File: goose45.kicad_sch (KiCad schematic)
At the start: 25 parts, among them SW1 Conn_01x02_Female, SW2 SW_Push, U1 STM32F103CBTx, X1 Crystal_GND24

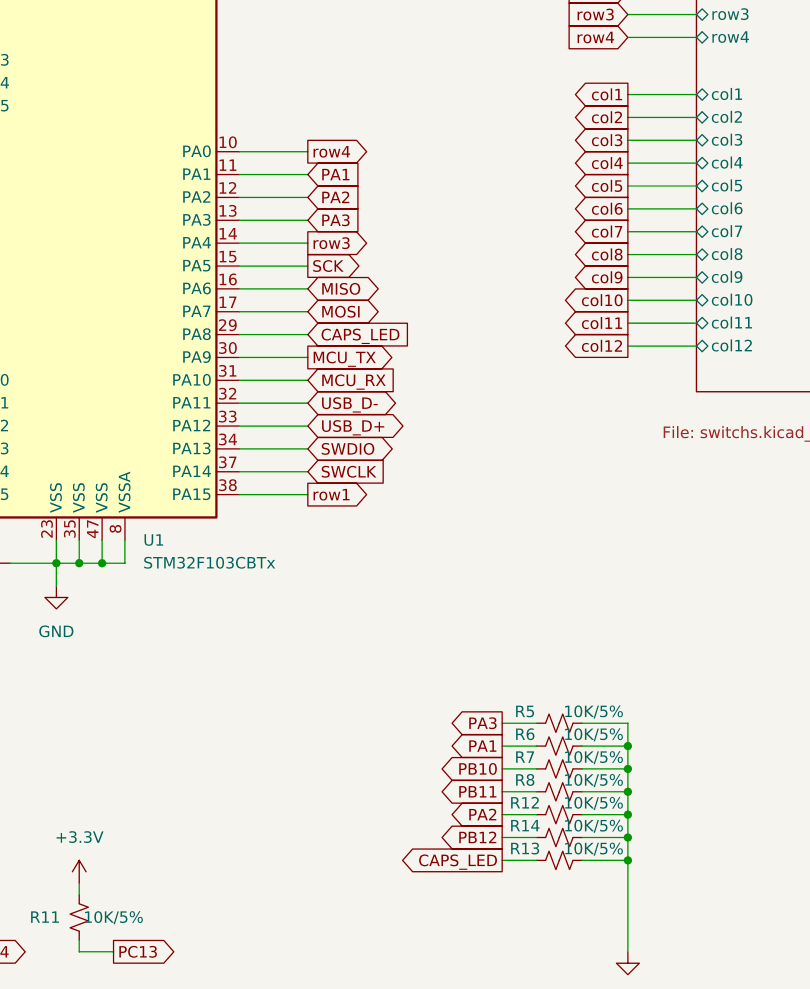
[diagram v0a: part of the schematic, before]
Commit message: update PCB layout
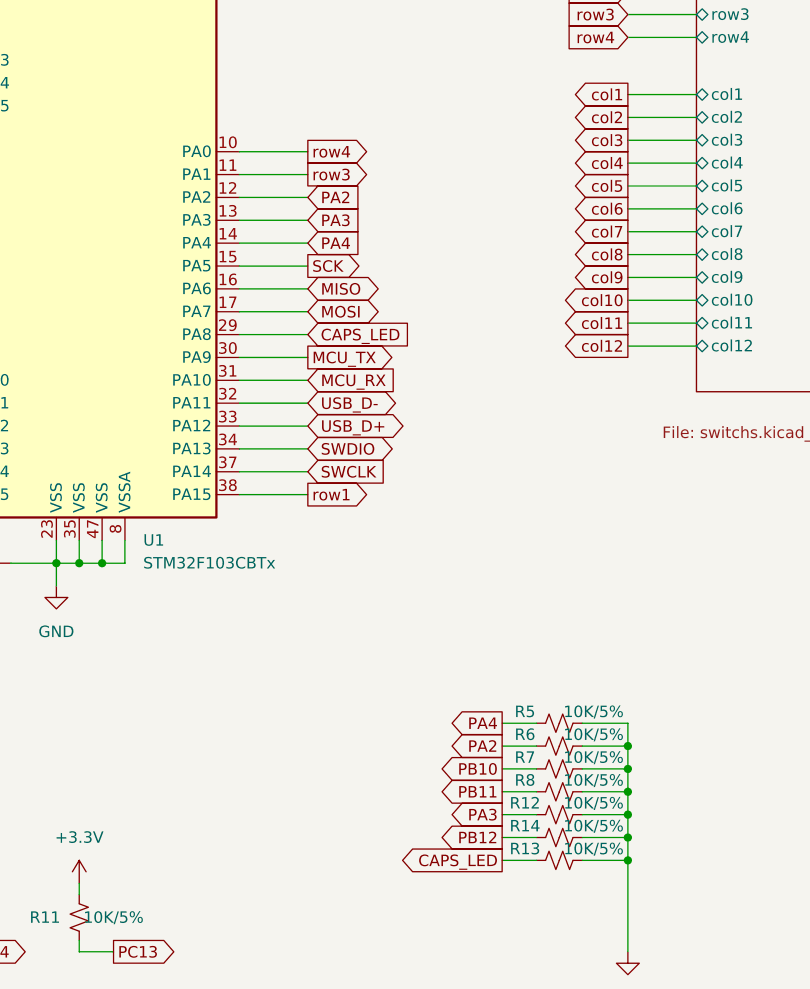
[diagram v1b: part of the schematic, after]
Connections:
- net PA2: now also R6.2; no longer R12.2
- net PA3: now also R12.2; no longer R5.2
- net row3: now also U1.11 (PA1); no longer U1.14 (PA4)
- removed net PA1: R6.2, U1.11 (PA1)
- new net PA4: R5.2, U1.14 (PA4)
